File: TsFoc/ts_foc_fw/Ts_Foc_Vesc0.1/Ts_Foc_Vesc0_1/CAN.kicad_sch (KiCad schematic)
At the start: 4 parts, among them U10 SIT1050TK, U11 SIT1050TK

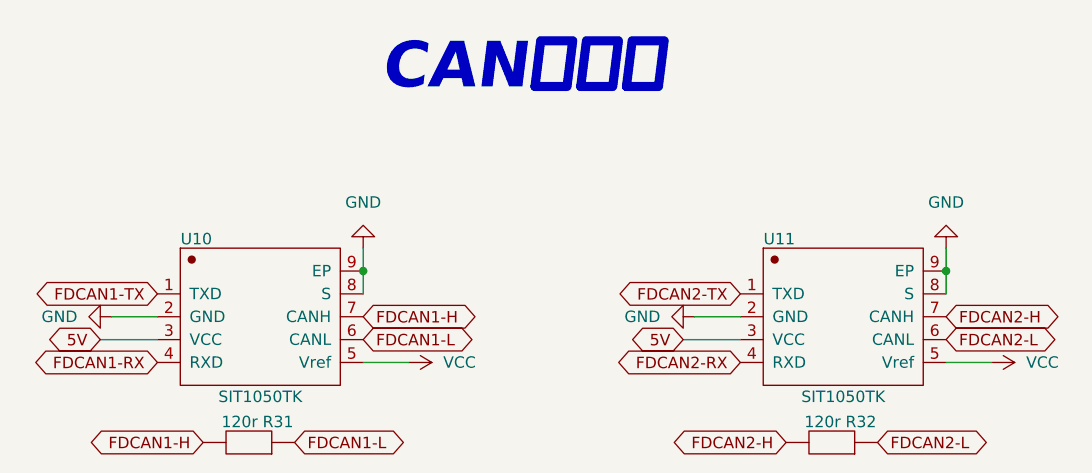
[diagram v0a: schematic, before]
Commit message: 第一版layout完成，准备打板验证
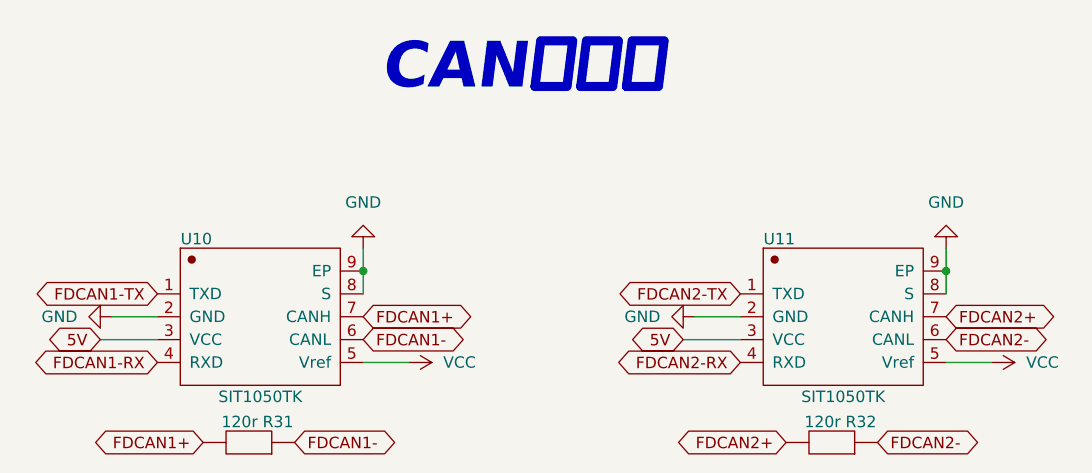
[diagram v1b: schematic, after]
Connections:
- net FDCAN1-H renamed FDCAN1+
- net FDCAN1-L renamed FDCAN1-
- net FDCAN2-H renamed FDCAN2+
- net FDCAN2-L renamed FDCAN2-
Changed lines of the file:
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@@
 		)
 	)
-	(global_label "FDCAN2-L"
+	(global_label "FDCAN2-"
 		(shape bidirectional)
 		(at 179.07 121.92 0)
@@
 		)
 		(property "Intersheetrefs" "${INTERSHEET_REFS}"
-			(at 193.0242 121.92 0)
+			(at 191.9961 121.92 0)
 			(effects
 				(font
@@
 		)
 	)
-	(global_label "FDCAN2-H"
+	(global_label "FDCAN2+"
 		(shape bidirectional)
 		(at 186.69 107.95 0)
@@
 		)
 		(property "Intersheetrefs" "${INTERSHEET_REFS}"
-			(at 200.9466 107.95 0)
+			(at 199.6161 107.95 0)
 			(effects
 				(font
@@
 		)
 	)
-	(global_label "FDCAN1-H"
+	(global_label "FDCAN1+"
 		(shape bidirectional)
 		(at 121.92 107.95 0)
@@
 		)
 		(property "Intersheetrefs" "${INTERSHEET_REFS}"
-			(at 136.1766 107.95 0)
+			(at 134.8461 107.95 0)
 			(effects
 				(font
@@
 		)
 	)
-	(global_label "FDCAN1-L"
+	(global_label "FDCAN1-"
 		(shape bidirectional)
 		(at 114.3 121.92 0)
@@
 		)
 		(property "Intersheetrefs" "${INTERSHEET_REFS}"
-			(at 128.2542 121.92 0)
-			(effects
-				(font
-					(size 1.27 1.27)
-				)
-				(justify left)
-				(hide yes)
-			)
-		)
-	)
-	(global_label "FDCAN1-H"
+			(at 127.2261 121.92 0)
+			(effects
+				(font
+					(size 1.27 1.27)
+				)
+				(justify left)
+				(hide yes)
+			)
+		)
+	)
+	(global_label "FDCAN1+"
 		(shape bidirectional)
 		(at 104.14 121.92 180)
@@
 		)
 		(property "Intersheetrefs" "${INTERSHEET_REFS}"
-			(at 89.8834 121.92 0)
-			(effects
-				(font
-					(size 1.27 1.27)
-				)
-				(justify right)
-				(hide yes)
-			)
-		)
-	)
-	(global_label "FDCAN1-L"
+			(at 91.2139 121.92 0)
+			(effects
+				(font
+					(size 1.27 1.27)
+				)
+				(justify right)
+				(hide yes)
+			)
+		)
+	)
+	(global_label "FDCAN1-"
 		(shape bidirectional)
 		(at 121.92 110.49 0)
@@
 		)
 		(property "Intersheetrefs" "${INTERSHEET_REFS}"
-			(at 135.8742 110.49 0)
+			(at 134.8461 110.49 0)
 			(effects
 				(font
@@
 		)
 	)
-	(global_label "FDCAN2-L"
+	(global_label "FDCAN2-"
 		(shape bidirectional)
 		(at 186.69 110.49 0)
@@
 		)
 		(property "Intersheetrefs" "${INTERSHEET_REFS}"
-			(at 200.6442 110.49 0)
+			(at 199.6161 110.49 0)
 			(effects
 				(font
@@
 		)
 	)
-	(global_label "FDCAN2-H"
+	(global_label "FDCAN2+"
 		(shape bidirectional)
 		(at 168.91 121.92 180)
@@
 		)
 		(property "Intersheetrefs" "${INTERSHEET_REFS}"
-			(at 154.6534 121.92 0)
-			(effects
-				(font
+			(at 155.9839 121.92 0)
+			(effects
+				(font
